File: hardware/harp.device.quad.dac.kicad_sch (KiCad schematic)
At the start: 0 parts

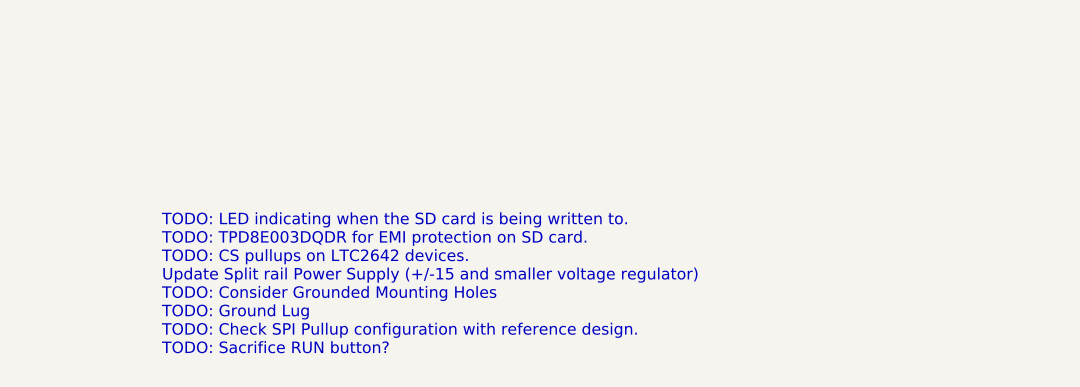
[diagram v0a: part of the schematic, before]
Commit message: update pcb draft
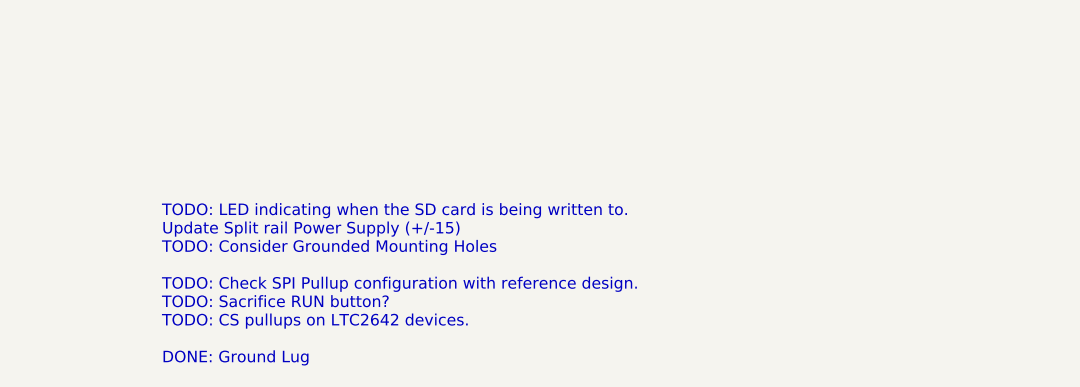
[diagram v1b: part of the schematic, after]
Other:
- note added: "TODO: LED indicating when the SD card is being written to. Update Split rail Power Supply (+/-15) TODO: Consider Grounded Mounting Holes TODO: Check SPI Pullup configuration with reference design. TODO: Sacrifice RUN button? TODO: CS pullups on LTC2642 devices. DONE: Ground Lug"
- note removed: "TODO: LED indicating when the SD card is being written to. TODO: TPD8E003DQDR for EMI protection on SD card. TODO: CS pullups on LTC2642 devices. Update Split rail Power Supply (+/-15 and smaller voltage regulator) TODO: Consider Grounded Mounting Holes TODO: Ground Lug TODO: Check SPI Pullup configuration with reference design. TODO: Sacrifice RUN button?"
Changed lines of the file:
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@@
 		(comment 1 "Hexabitz")
 	)
-	(text "TODO: LED indicating when the SD card is being written to.\nTODO: TPD8E003DQDR for EMI protection on SD card.\nTODO: CS pullups on LTC2642 devices.\nUpdate Split rail Power Supply (+/-15 and smaller voltage regulator)\nTODO: Consider Grounded Mounting Holes\nTODO: Ground Lug\nTODO: Check SPI Pullup configuration with reference design.\nTODO: Sacrifice RUN button?"
+	(text "TODO: LED indicating when the SD card is being written to.\nUpdate Split rail Power Supply (+/-15)\nTODO: Consider Grounded Mounting Holes\n\nTODO: Check SPI Pullup configuration with reference design.\nTODO: Sacrifice RUN button?\nTODO: CS pullups on LTC2642 devices.\n\nDONE: Ground Lug"
 		(exclude_from_sim no)
 		(at 96.012 127.254 0)
